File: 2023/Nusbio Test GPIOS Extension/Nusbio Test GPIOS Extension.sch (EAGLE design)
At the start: 7 parts

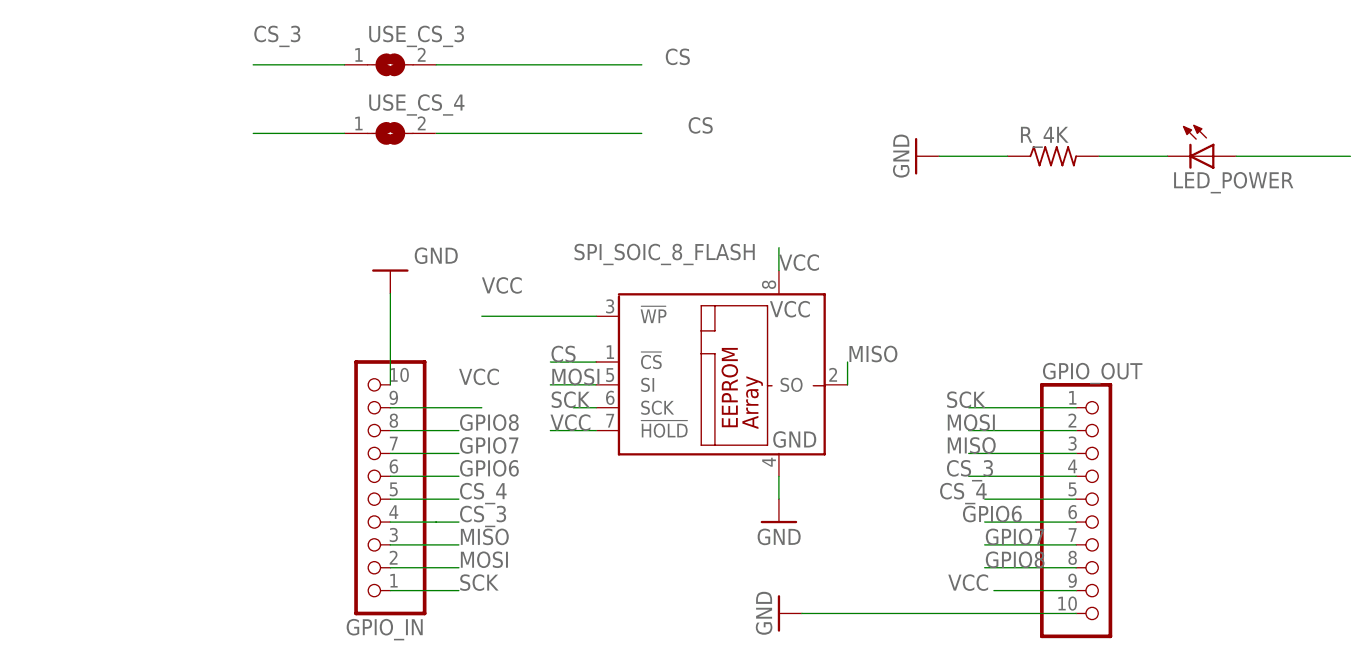
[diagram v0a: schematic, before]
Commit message: Test Esxtension
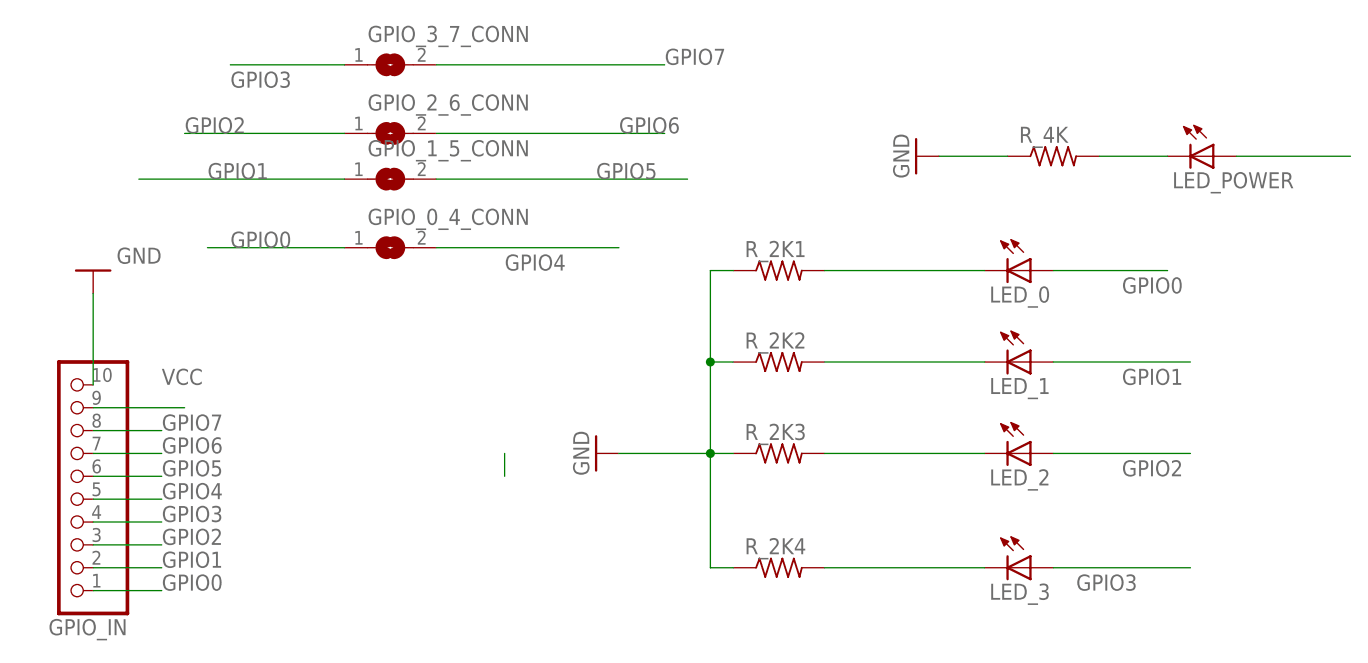
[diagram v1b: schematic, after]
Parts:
- removed GPIO_OUT: PINHD-1X10, adafruit:PINHD-1X10
- removed SPI_SOIC_8_FLASH: 25AA080SN, microchip:25AA080SN
- added GPIO_0_4_CONN, GPIO_1_5_CONN: (no value), microbuilder:SOLDERJUMPERREFLOW
- added LED_0, LED_1, LED_2, LED_3: (no value), adafruit:LEDSMT1206
- added R_2K1, R_2K2, R_2K3, R_2K4: (no value), adafruit:R-US_R1206
- renumbered USE_CS_3 to GPIO_3_7_CONN, USE_CS_4 to GPIO_2_6_CONN
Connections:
- removed net CS: GPIO_2_6_CONN.2, GPIO_3_7_CONN.2, SPI_SOIC_8_FLASH.!CS
- removed net CS_3: GPIO_3_7_CONN.1, GPIO_IN.4, GPIO_OUT.4
- removed net CS_4: GPIO_2_6_CONN.1, GPIO_IN.5, GPIO_OUT.5
- removed net GPIO8: GPIO_IN.8, GPIO_OUT.8
- removed net MISO: GPIO_IN.3, GPIO_OUT.3, SPI_SOIC_8_FLASH.SO
- removed net MOSI: GPIO_IN.2, GPIO_OUT.2, SPI_SOIC_8_FLASH.SI
- removed net SCK: GPIO_IN.1, GPIO_OUT.1, SPI_SOIC_8_FLASH.SCK
- new net GPIO0: GPIO_0_4_CONN.1, GPIO_IN.1, LED_0.A
- new net GPIO1: GPIO_1_5_CONN.1, GPIO_IN.2, LED_1.A
- new net GPIO2: GPIO_2_6_CONN.1, GPIO_IN.3, LED_2.A
- new net GPIO3: GPIO_3_7_CONN.1, GPIO_IN.4, LED_3.A
- new net GPIO4: GPIO_0_4_CONN.2, GPIO_IN.5
- new net GPIO5: GPIO_1_5_CONN.2, GPIO_IN.6
- new net N$1: LED_0.C, R_2K1.2
- new net N$3: LED_1.C, R_2K2.2
- new net N$4: LED_2.C, R_2K3.2
- new net N$5: LED_3.C, R_2K4.2
- net GND: now also R_2K1.1, R_2K2.1, R_2K3.1, R_2K4.1; no longer GPIO_OUT.10, SPI_SOIC_8_FLASH.GND
- net GPIO6: now also GPIO_2_6_CONN.2, GPIO_IN.7; no longer GPIO_IN.6, GPIO_OUT.6
- net GPIO7: now also GPIO_3_7_CONN.2, GPIO_IN.8; no longer GPIO_IN.7, GPIO_OUT.7
- net VCC: no longer GPIO_OUT.9, SPI_SOIC_8_FLASH.!HOLD, SPI_SOIC_8_FLASH.!WP, SPI_SOIC_8_FLASH.VCC
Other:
- moved on the sheet: GPIO_IN
